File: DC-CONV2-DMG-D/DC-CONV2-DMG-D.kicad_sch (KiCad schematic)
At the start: 26 parts, among them J1 Conn_01x04, Q1 2SD1664R, Q2 2SC2412, Q3 DTC143T, Q4 DTC143T, Q5 DTC143T, T1 280

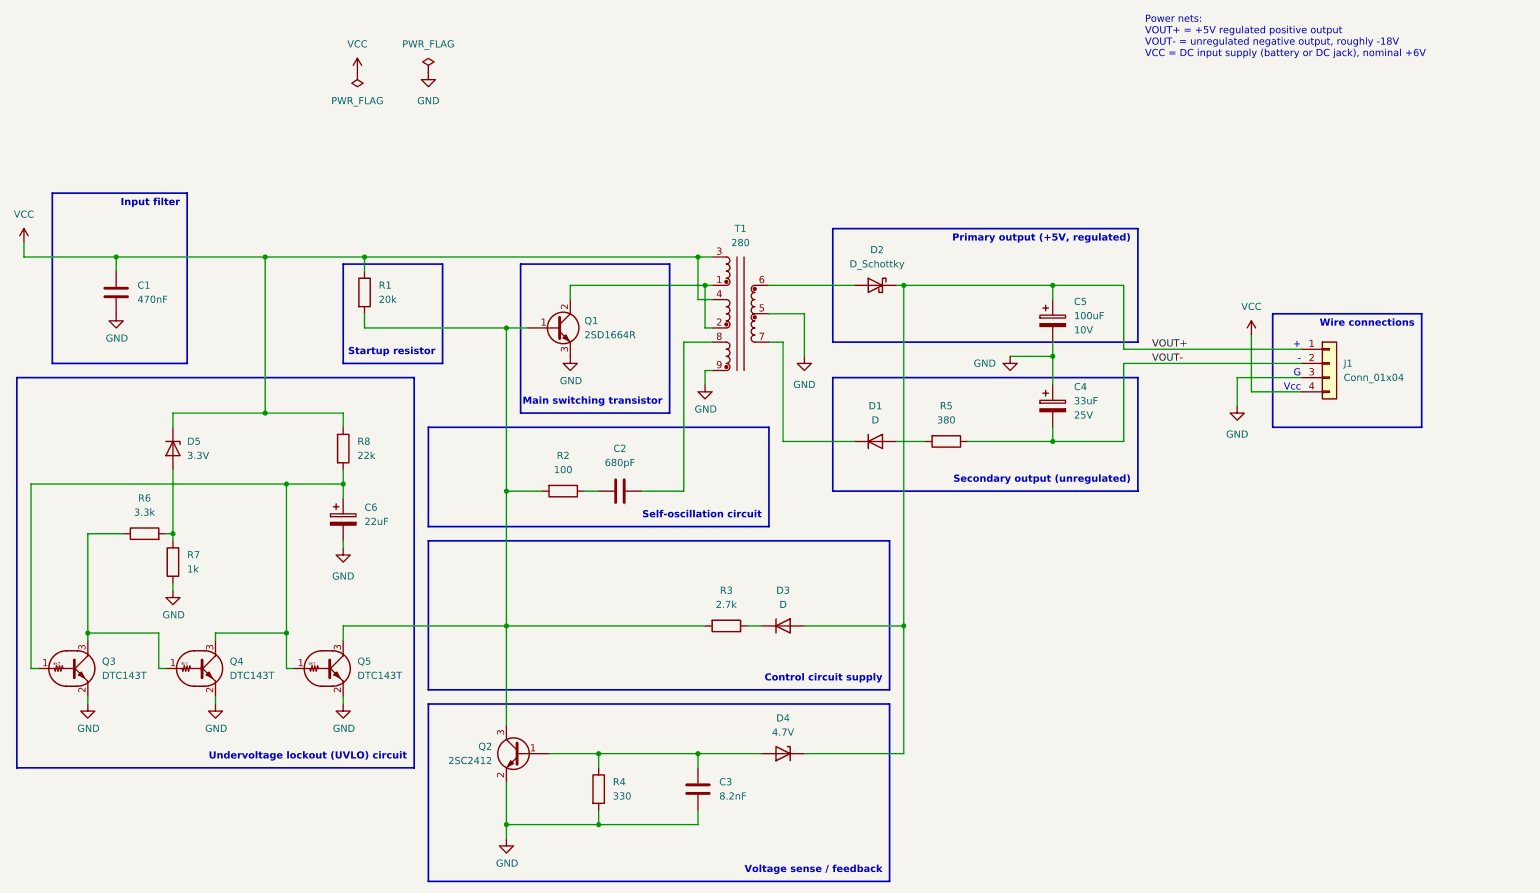
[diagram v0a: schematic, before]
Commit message: Update to latest KiCad
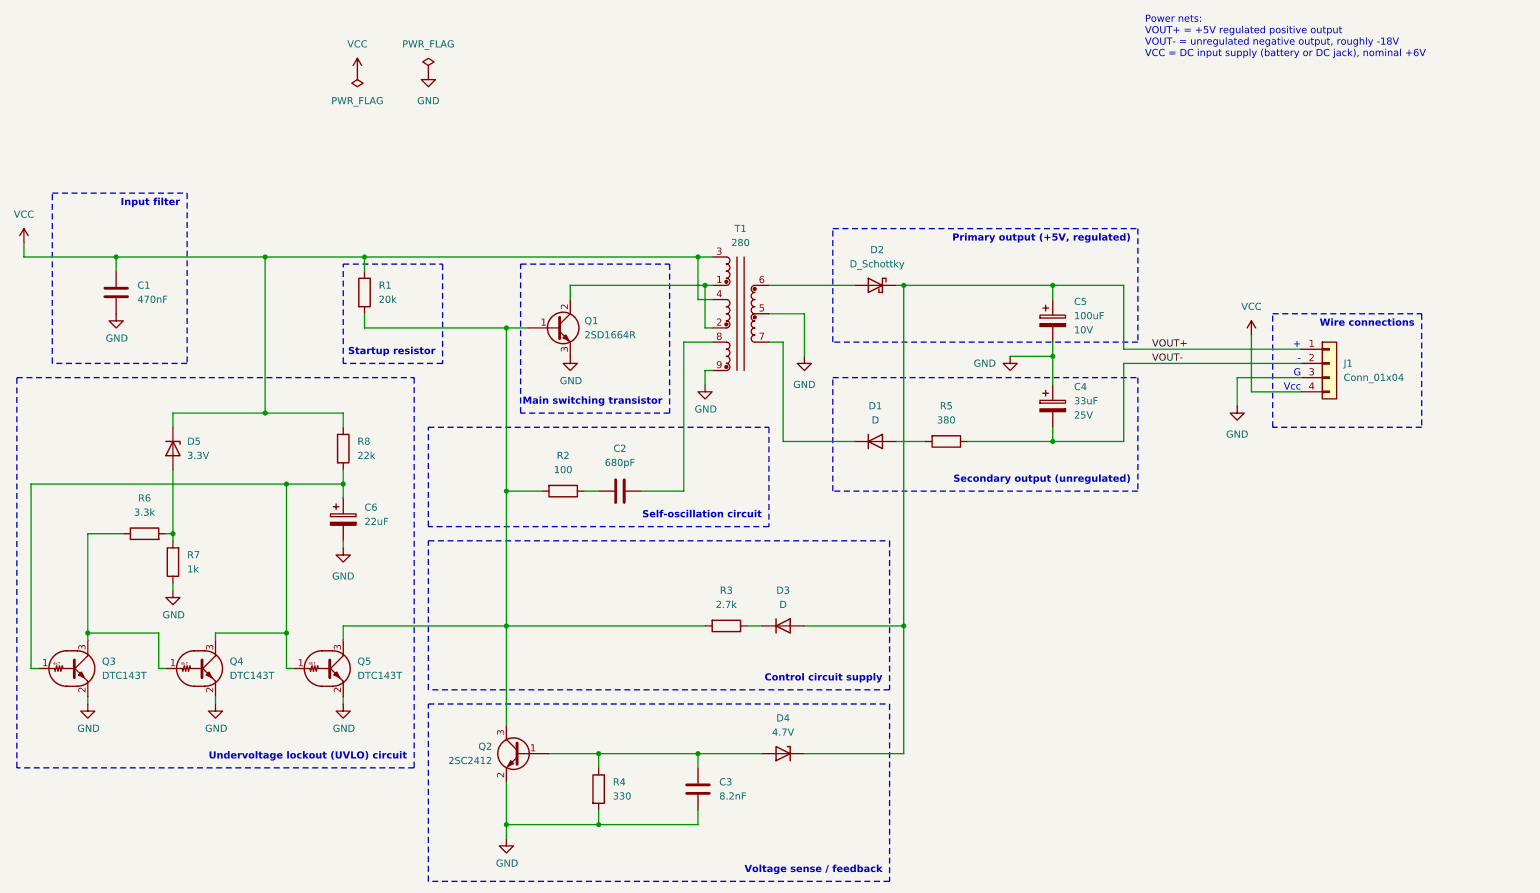
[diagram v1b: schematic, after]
